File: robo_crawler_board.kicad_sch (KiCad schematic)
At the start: 13 parts, among them J1 Screw_Terminal_01x02, J2 Screw_Terminal_01x02, J3 Screw_Terminal_01x02, U4 DRV8871DDA, U5 DRV8871DDA

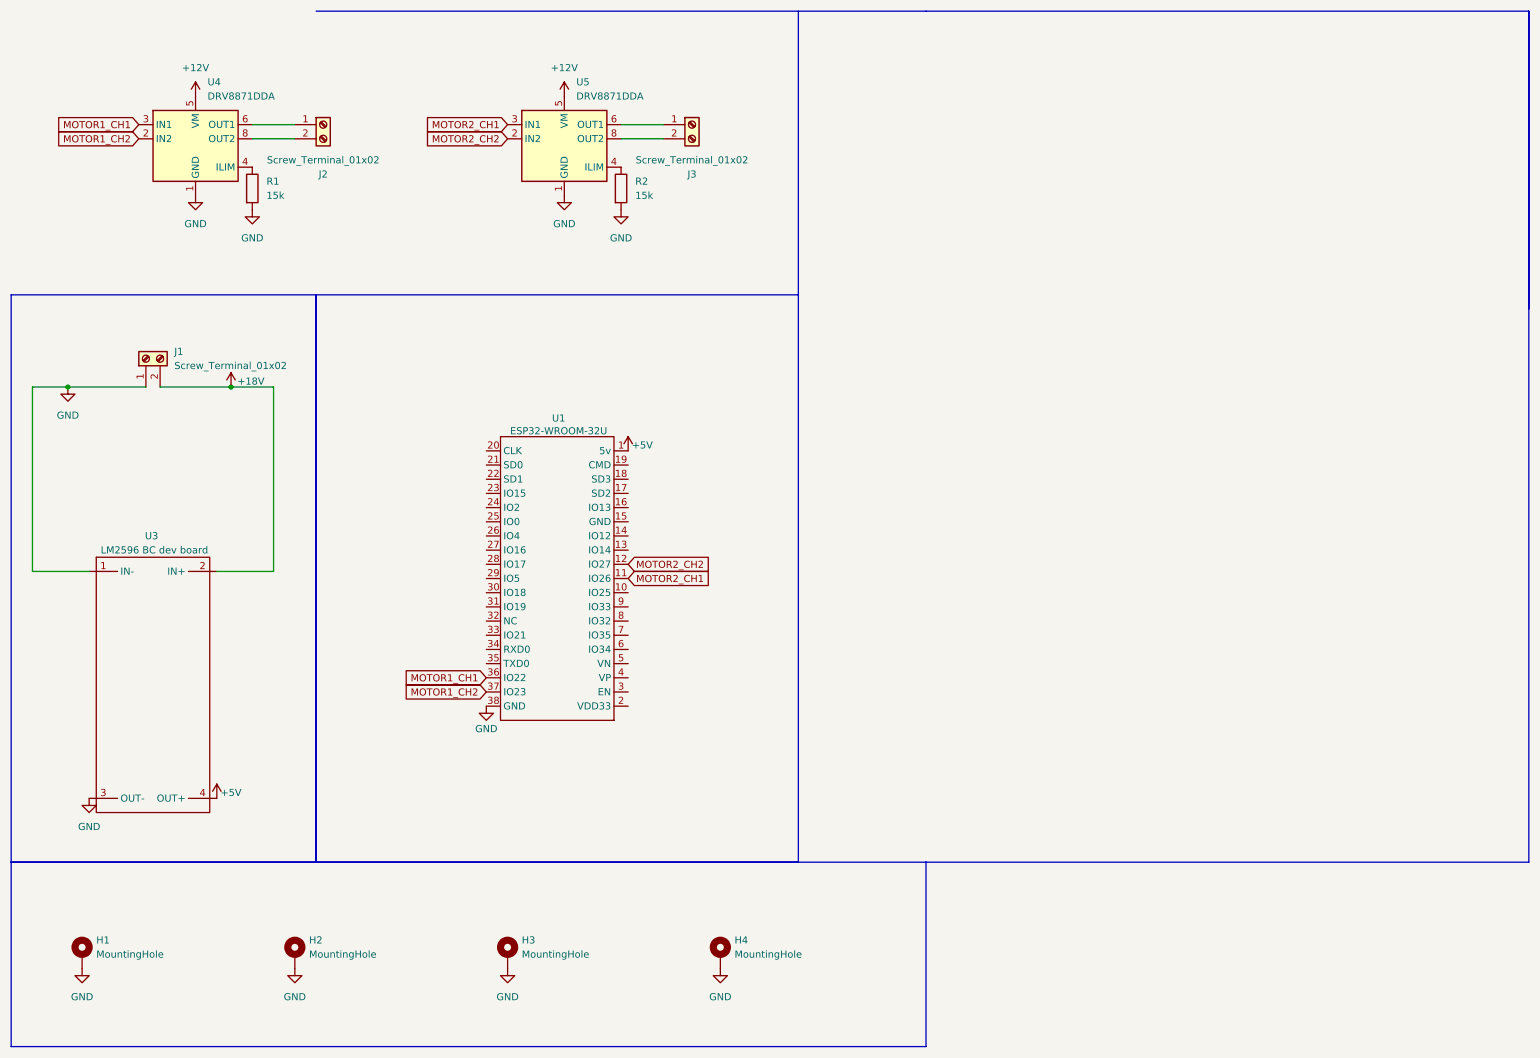
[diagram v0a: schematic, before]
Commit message: saving progress
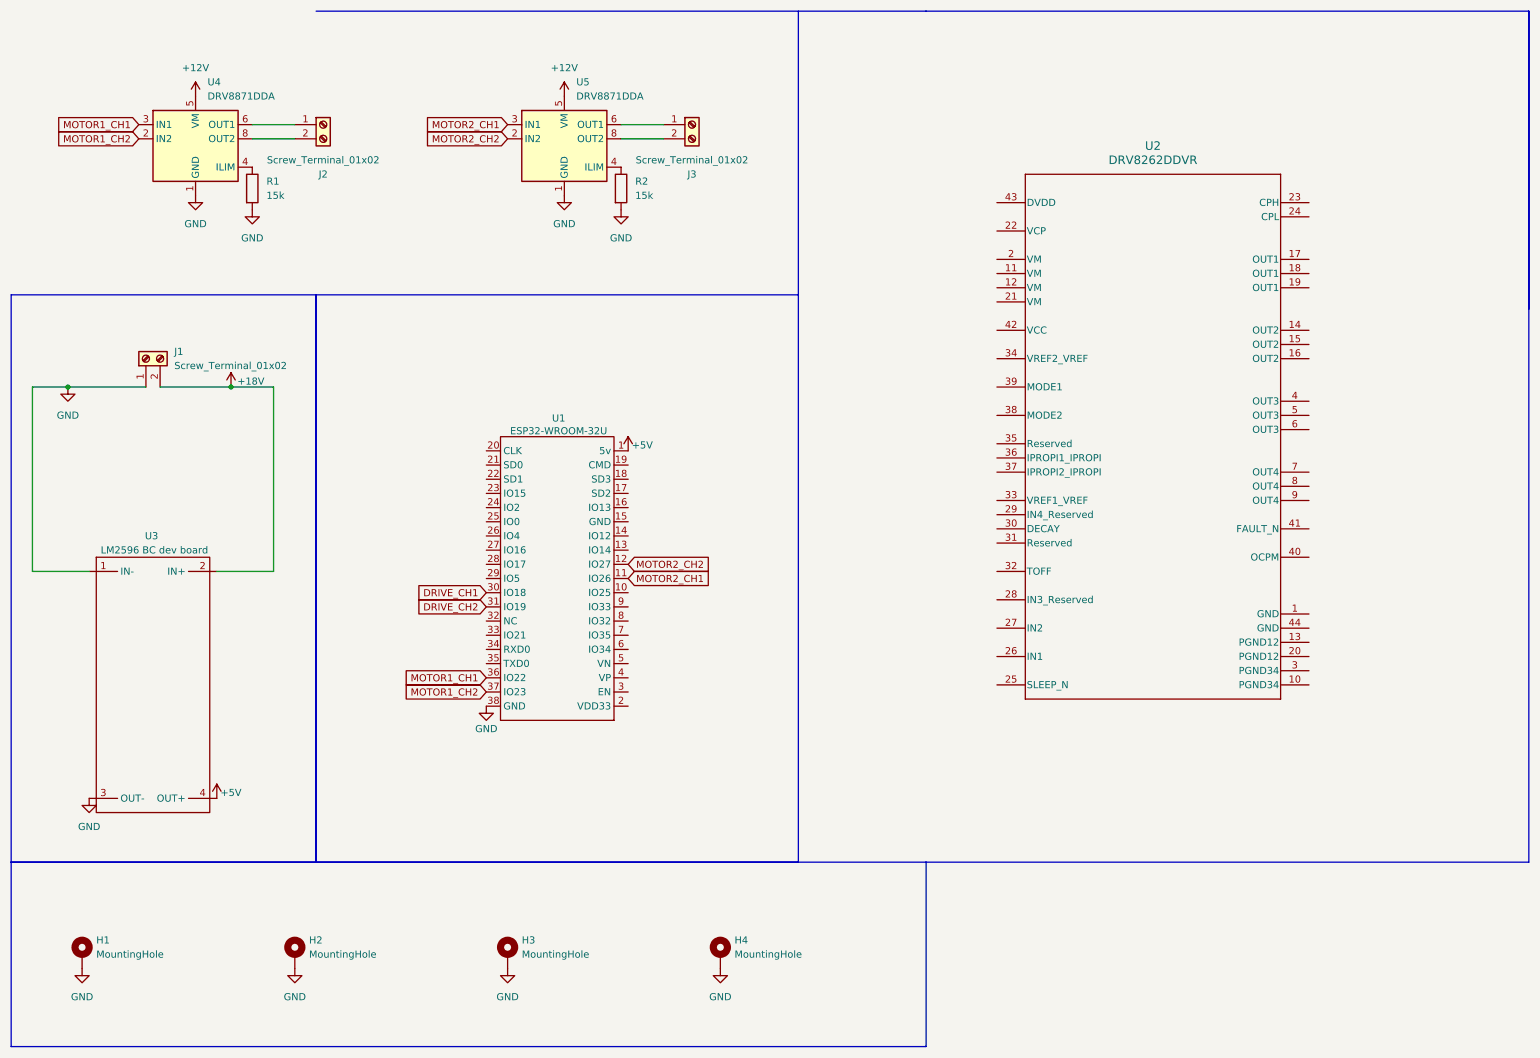
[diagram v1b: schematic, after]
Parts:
- added U2: DRV8262DDVR, DDV0044E-IPC_A, symbol DRV8262DDVR:DRV8262DDVR
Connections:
- net DRIVE_CH1: now reaches U1.30 (IO18)
- net DRIVE_CH2: now reaches U1.31 (IO19)
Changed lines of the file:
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@@
+		)
+	)
+	(global_label "DRIVE_CH1"
+		(shape input)
+		(at 97.79 116.84 180)
+		(fields_autoplaced yes)
+		(effects
+			(font
+				(size 1.27 1.27)
+			)
+			(justify right)
+		)
+		(property "Intersheetrefs" "${INTERSHEET_REFS}"
+			(at 84.6448 116.84 0)
+			(effects
+				(font
+					(size 1.27 1.27)
+				)
+				(justify right)
+				(hide yes)
+			)
+		)
+	)
+	(global_label "DRIVE_CH2"
+		(shape input)
+		(at 97.79 119.38 180)
+		(fields_autoplaced yes)
+		(effects
+			(font
+				(size 1.27 1.27)
+			)
+			(justify right)
+		)
+		(property "Intersheetrefs" "${INTERSHEET_REFS}"
+			(at 84.6448 119.38 0)
+			(effects
+				(font
+					(size 1.27 1.27)
+				)
+				(justify right)
+				(hide yes)
+			)
 		)
 	)
@@
 					(unit 1)
 				)
+			)
+		)
+	)
+	(symbol
+		(lib_id "DRV8262DDVR:DRV8262DDVR")
+		(at 189.23 46.99 0)
+		(unit 1)
+		(exclude_from_sim no)
+		(in_bom yes)
+		(on_board yes)
+		(dnp no)
+		(fields_autoplaced yes)
+		(property "Reference" "U2"
+			(at 217.17 36.83 0)
+			(effects
+				(font
+					(size 1.524 1.524)
+				)
+			)
+		)
+		(property "Value" "DRV8262DDVR"
+			(at 217.17 39.37 0)
+			(effects
+				(font
+					(size 1.524 1.524)
+				)
+			)
+		)
+		(property "Footprint" "DDV0044E-IPC_A"
+			(at 189.23 46.99 0)
+			(effects
+				(font
+					(size 1.27 1.27)
+					(italic yes)
+				)
+				(hide yes)
+			)
+		)
+		(property "Datasheet" "https://www.ti.com/lit/gpn/drv8262"
+			(at 189.23 46.99 0)
+			(effects
+				(font
+					(size 1.27 1.27)
+					(italic yes)
+				)
+				(hide yes)
+			)
+		)
+		(property "Description" ""
+			(at 189.23 46.99 0)
+			(effects
+				(font
+					(size 1.27 1.27)
+				)
+				(hide yes)
+			)
+		)
+		(pin "23"
+		)
+		(pin "22"
+		)
+		(pin "33"
+		)
+		(pin "11"
+		)
+		(pin "42"
+		)
+		(pin "38"
+		)
+		(pin "37"
+		)
+		(pin "2"
+		)
+		(pin "12"
+		)
+		(pin "21"
+		)
+		(pin "30"
+		)
+		(pin "34"
+		)
+		(pin "36"
+		)
+		(pin "35"
+		)
+		(pin "31"
+		)
+		(pin "43"
+		)
+		(pin "39"
+		)
+		(pin "32"
+		)
+		(pin "27"
+		)
+		(pin "26"
+		)
+		(pin "29"
+		)
+		(pin "25"
+		)
+		(pin "28"
+		)
+		(pin "20"
+		)
+		(pin "10"
+		)
+		(pin "17"
+		)
+		(pin "18"
+		)
+		(pin "13"
+		)
+		(pin "16"
+		)
+		(pin "6"
+		)
+		(pin "8"
+		)
+		(pin "9"
+		)
+		(pin "41"
+		)
+		(pin "1"
+		)
+		(pin "4"
+		)
+		(pin "19"
+		)
+		(pin "5"
+		)
+		(pin "40"
+		)
+		(pin "24"
+		)
+		(pin "15"
+		)
+		(pin "14"
+		)
+		(pin "7"
+		)
+		(pin "44"
+		)
+		(pin "3"
+		)
+		(instances
+			(project ""
+				(path "/8c23940b-1549-4d4e-a5eb-1280177a037e"
+					(reference "U2")
+					(unit 1)
+				)
